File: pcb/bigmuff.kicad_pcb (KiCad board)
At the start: 2 copper layers, 120 x 90 mm, 70 parts, among them J1 NRJ4HF, J10 Conn_01x02_Pin, J11 Conn_01x02_Pin, J2 NRJ4HF, J3 Conn_01x02_Pin, J4 Barrel_Jack_Switch, J5 Conn_01x02_Pin, J6 Conn_01x02_Pin, J7 Conn_01x02_Pin, J8 Conn_01x02_Pin, J9 Conn_01x02_Pin, Q1 BC549, Q2 BC549, Q3 BC549, Q4 BC549

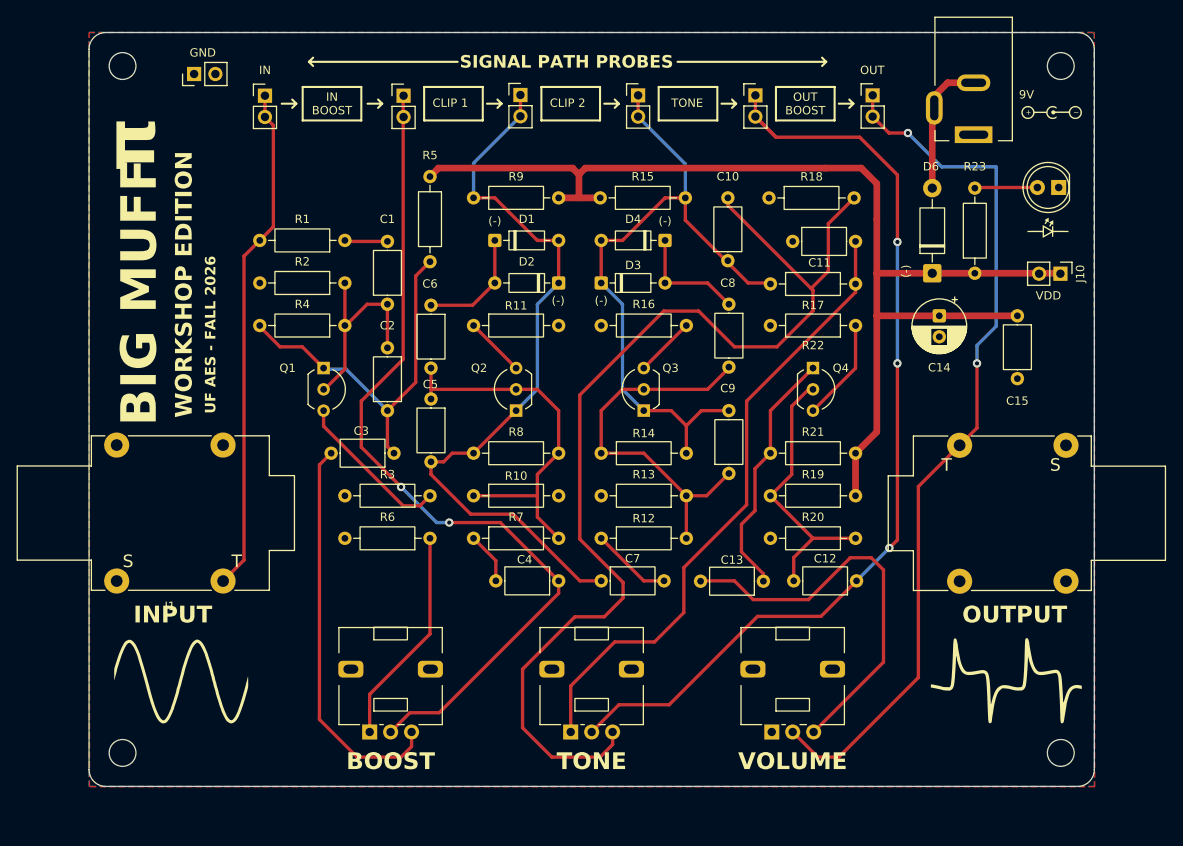
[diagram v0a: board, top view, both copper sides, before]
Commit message: pre fab update 2
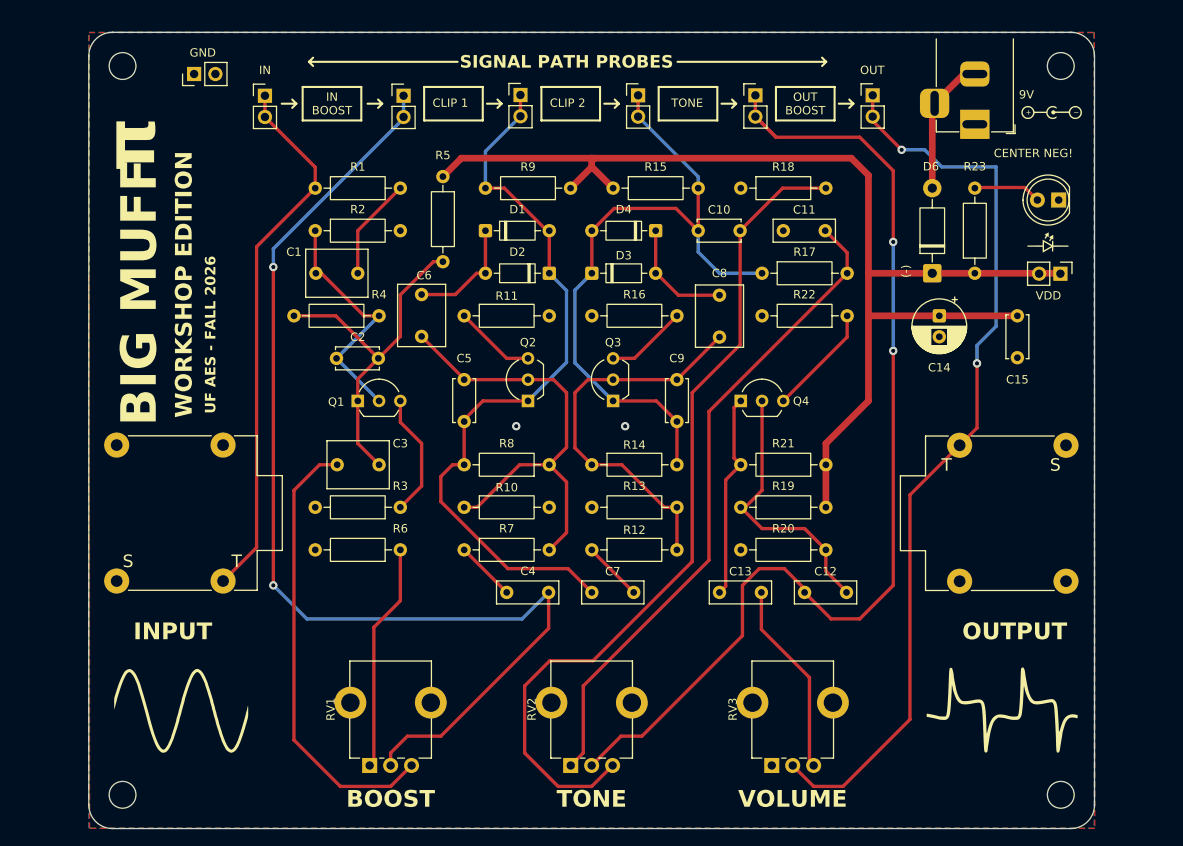
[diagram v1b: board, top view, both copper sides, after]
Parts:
- added G***: LOGO, LOGO, B.Cu at (143.5, 86.2)
- C1, C3, C6, C8: footprint Capacitor_THT:C_Axial_L5.1mm_D3.1mm_P7.50mm_Horizontal -> Capacitor_THT:C_Rect_L7.2mm_W5.5mm_P5.00mm_FKS2_FKP2_MKS2_MKP2
- C10: value 4nF -> 3.9nF; footprint Capacitor_THT:C_Axial_L5.1mm_D3.1mm_P7.50mm_Horizontal -> Capacitor_THT:C_Disc_D5.0mm_W2.5mm_P5.00mm
- C11, C12, C13, C4, C7: footprint Capacitor_THT:C_Axial_L5.1mm_D3.1mm_P7.50mm_Horizontal -> Capacitor_THT:C_Rect_L7.2mm_W2.5mm_P5.00mm_FKS2_FKP2_MKS2_MKP2
- C15, C2, C5, C9: footprint Capacitor_THT:C_Axial_L5.1mm_D3.1mm_P7.50mm_Horizontal -> Capacitor_THT:C_Disc_D5.0mm_W2.5mm_P5.00mm
- J1, J2: value NRJ4HF -> NMJ4HFD2; footprint Connector_Audio:Jack_6.35mm_Neutrik_NMJ4HFD3_Horizontal -> Connector_Audio:Jack_6.35mm_Neutrik_NMJ4HFD2_Horizontal
- J4: footprint Connector_BarrelJack:BarrelJack_Kycon_KLDX-0202-xC_Horizontal -> bigmuff:BarrelJack_Tayda_A-4118_Horizontal
- RV1, RV2, RV3: footprint Potentiometer_THT:Potentiometer_Alps_RK09L_Single_Vertical -> bigmuff:Potentiometer_Alpha_RD901F-40-00D_RoundLegs
- moved C9 12.8 mm to (170.2, 91.4), turned to -90 degrees
- moved Q4 9.47 mm to (177.8, 94.0), turned to 0 degrees
- moved C1 9.31 mm to (127.1, 78.7), turned to 0 degrees
- moved R1 9.10 mm to (137.2, 68.6)
- moved R2 7.17 mm to (127.0, 73.7), turned to 0 degrees
- moved C12 6.35 mm to (185.4, 116.8), turned to 0 degrees
- moved C2 6.21 mm to (129.5, 88.9), turned to 0 degrees
- moved Q1 5.66 mm to (132.1, 94.0), turned to 0 degrees
- moved C13 5.41 mm to (175.3, 116.8), turned to 0 degrees
- moved C10 5.03 mm to (172.7, 73.7), turned to 0 degrees
- moved H3 5.00 mm to (216.0, 141.0)
- moved H4 5.00 mm to (104.0, 141.0)
- moved C5 4.58 mm to (144.8, 91.4)
- moved R4 4.24 mm to (134.6, 83.8)
- moved RV1 4.00 mm to (133.5, 137.5)
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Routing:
- net BOOST_OUT: track 103.2 -> 131.5 mm
- net Net-(C10-Pad2): track 129.4 -> 101.6 mm
- net Net-(C13-Pad2): track 48.3 -> 23.2 mm
- net TONE_OUT: track 115.4 -> 128.3 mm, vias 3 -> 2
- net Net-(Q2-B): track 44.9 -> 53.7 mm
- net Net-(C1-Pad2): track 5.13 -> 12.3 mm
- net Net-(C3-Pad2): track 47.5 -> 53.6 mm
- net Net-(Q4-C): track 30.1 -> 24.6 mm
- net Net-(Q1-E): track 19.0 -> 14.8 mm
- net IN: track 60.8 -> 65.0 mm
- net VDD: track 140.1 -> 144.1 mm
- net Net-(Q1-B): track 25.2 -> 29.1 mm
- net OUT: track 104.7 -> 108.6 mm
- net Net-(C11-Pad2): track 75.4 -> 78.6 mm
- net Net-(Q2-E): track 7.18 -> 9.72 mm
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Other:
- board size 120 x 90 mm -> 120.1 x 95.1 mm
- board text added: "Bill Of Materials"
- board text added: "CENTER NEG!"
- board text added: "EVAN GEHLER"
- board text added: "RESISTORS 100: R3 150: R11 R16 1k: R6 3.3k: R22 4.7k: R23 10k: R5 R7 R9 R12 R15 15k: R21 22k: R18 33k: R1 R17 47k: R2 100k: R10 R13 R20 430k: R19 470k: R4 R8 R14 CAPACITORS 470p: C2 C5 C9 3.9n: C10 10n: C11 100n film: C4 C7 C12 C13 100n cer: C15 1u film: C1 C3 C6 C8 100u 25V: C14 (pol) SEMICONDUCTORS 1N4148: D1-D4 1N5817: D6 LED: D5 BC549C: Q1-Q4 POTS B100k"
- board text added: "UF AES WORLDWIDE"
- board text added: "github.com/ufaes/BigMuff"
